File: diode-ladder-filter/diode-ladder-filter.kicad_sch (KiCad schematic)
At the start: 67 parts, among them J1 Input, J2 CV1, J3 CV2, J4 Output, J5 Power, J6 Power, J7 Power, SW1 LPF, SW2 Resonance_safety, SW3 BPF, SW4 HPF, U1 TL074, U2 TL074

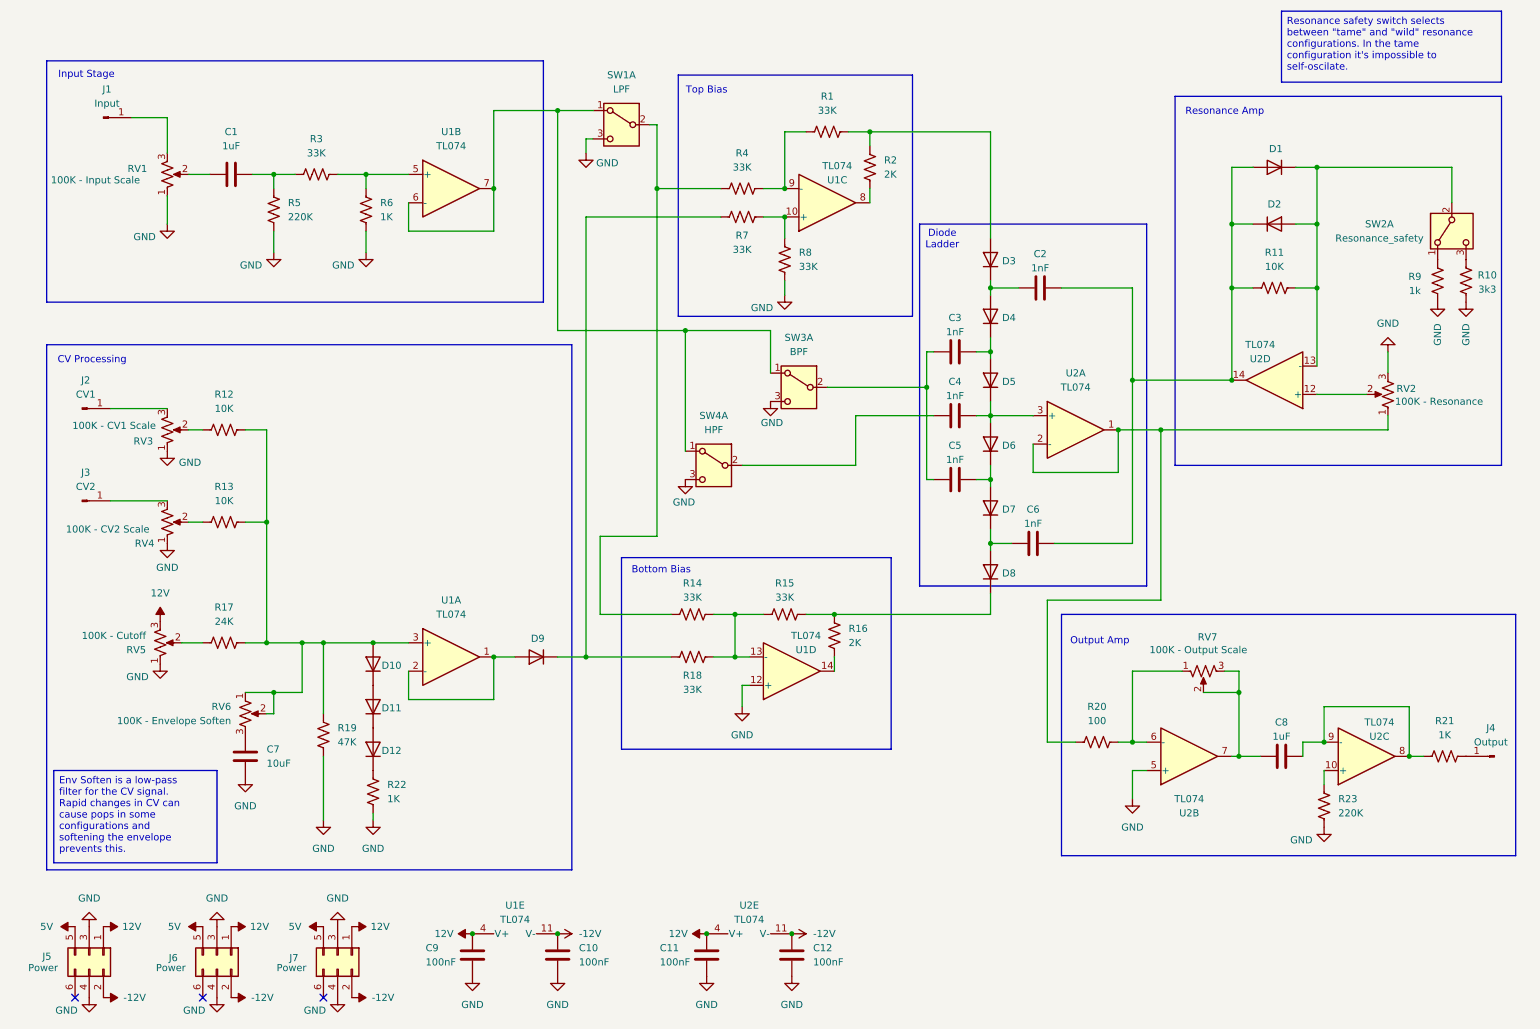
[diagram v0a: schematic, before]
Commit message: Update some modules
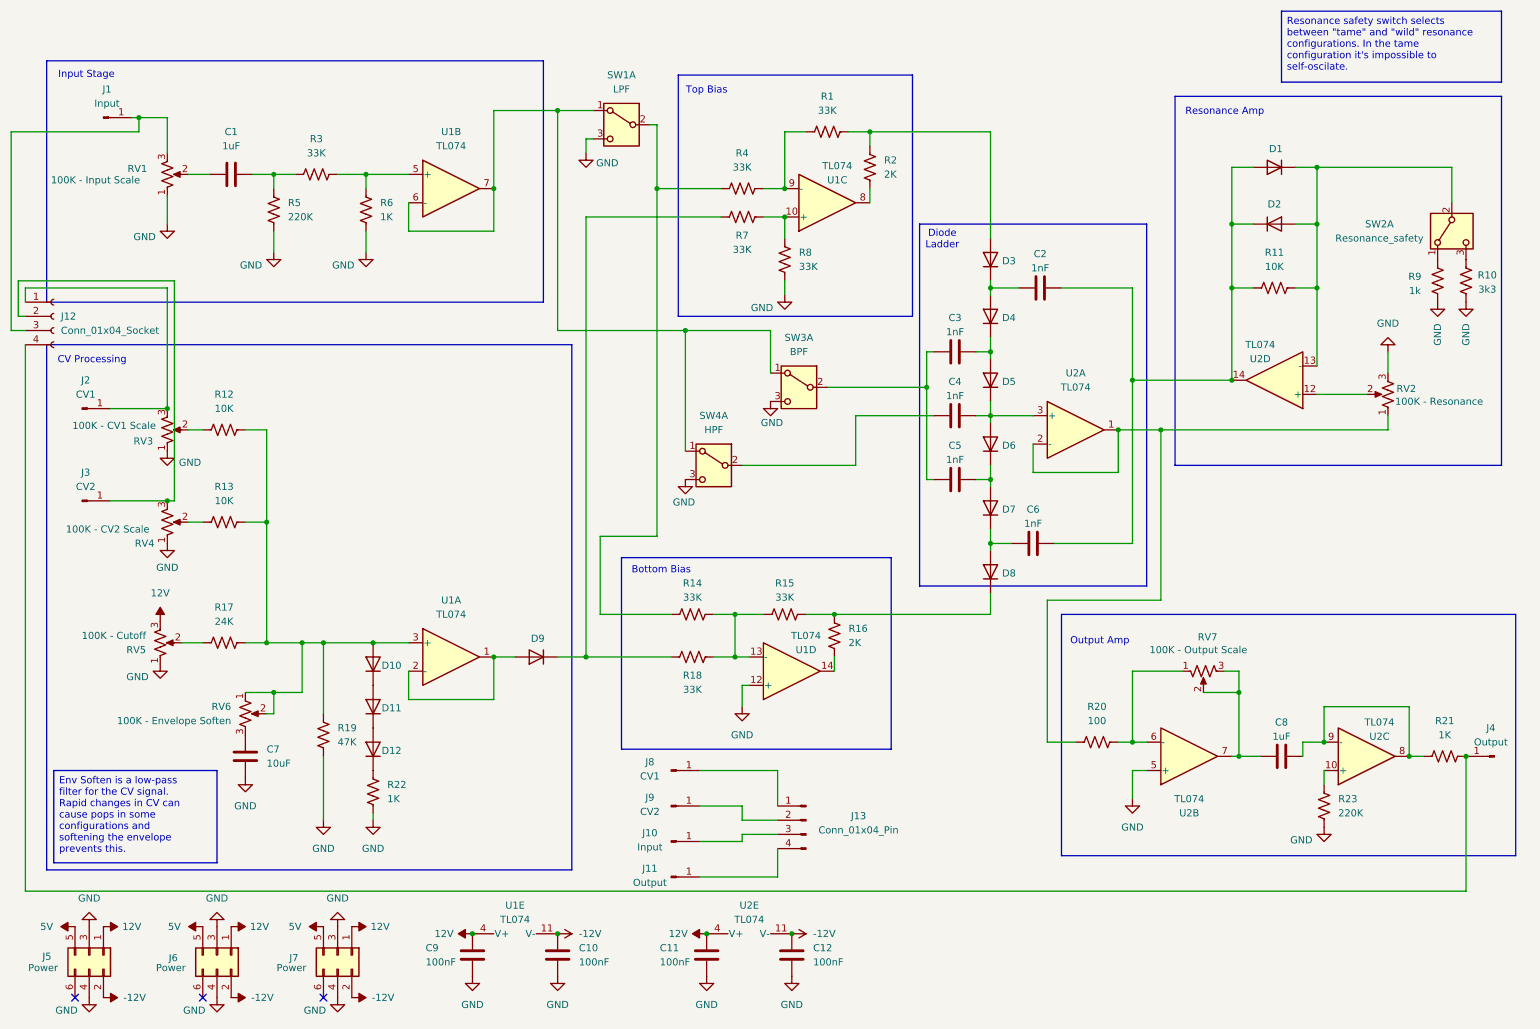
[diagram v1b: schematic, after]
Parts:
- added J10: Input, modular2:banana-jack, symbol Connector:Conn_01x01_Pin
- added J11: Output, modular2:banana-jack, symbol Connector:Conn_01x01_Pin
- added J12: Conn_01x04_Socket, Connector_PinSocket_2.54mm:PinSocket_1x04_P2.54mm_Vertical, symbol Connector:Conn_01x04_Socket
- added J13: Conn_01x04_Pin, Connector_PinHeader_2.54mm:PinHeader_1x04_P2.54mm_Vertical, symbol Connector:Conn_01x04_Pin
- added J8: CV1, modular2:banana-jack, symbol Connector:Conn_01x01_Pin
- added J9: CV2, modular2:banana-jack, symbol Connector:Conn_01x01_Pin
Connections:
- net at J3.1 (Pin_1), RV4.3: now also J12.2 (Pin_2)
- net at J4.1 (Pin_1), R21.2: now also J12.4 (Pin_4)
- net at J2.1 (Pin_1), RV3.3: now also J12.1 (Pin_1)
- net at J1.1 (Pin_1), RV1.3: now also J12.3 (Pin_3)
- new net: J10.1 (Pin_1), J13.3 (Pin_3)
- new net: J13.1 (Pin_1), J8.1 (Pin_1)
- new net: J11.1 (Pin_1), J13.4 (Pin_4)
- new net: J13.2 (Pin_2), J9.1 (Pin_1)
